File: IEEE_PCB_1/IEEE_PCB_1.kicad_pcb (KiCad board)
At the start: 2 copper layers, 89.3 x 109 mm, 28 parts, among them SW1 EG1218, U1 555, U2 4017

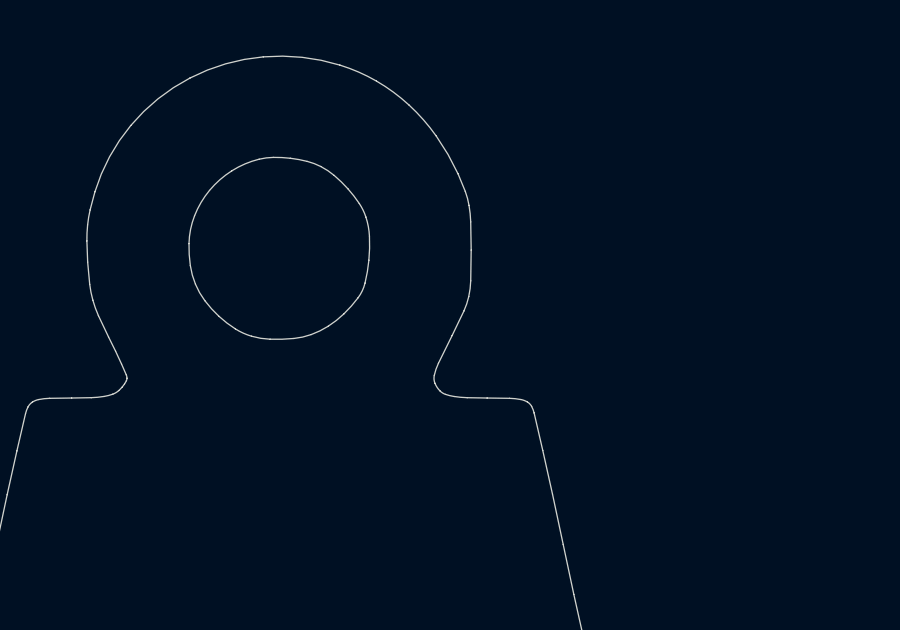
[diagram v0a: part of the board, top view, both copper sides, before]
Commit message: Demo(Test)
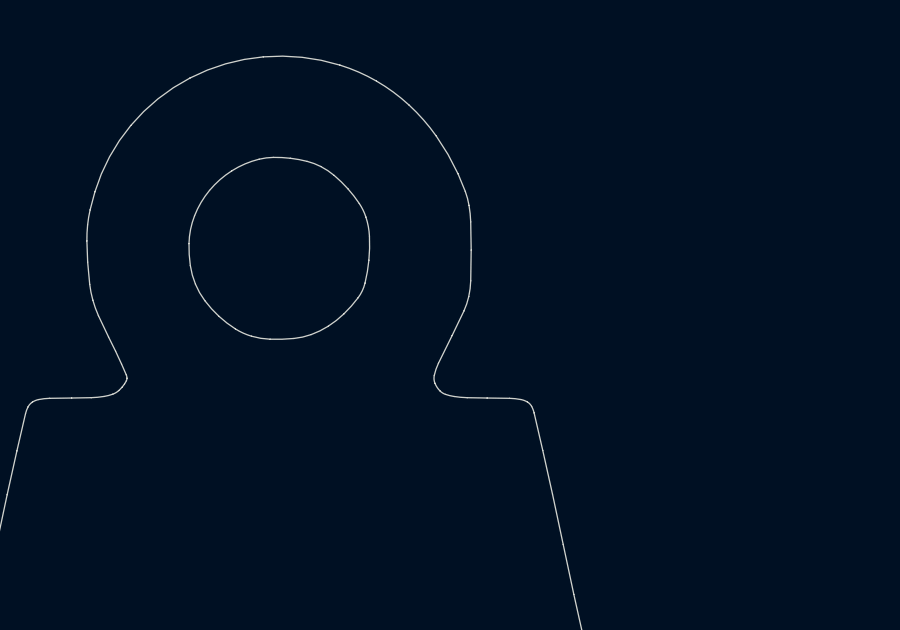
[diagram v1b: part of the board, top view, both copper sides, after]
